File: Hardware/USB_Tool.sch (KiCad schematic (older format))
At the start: 57 parts, among them J1 USB_B_Micro, P1 RED, P2 RGB, P3 Green, P4 Green, P5 Blue, P6 Green, P7 Green, P8 Blue, SW1 SW_2TO1, U1 MRF89XAM8A, U2 NCP114, U3 MCP2221A, U4 PIC18F46K40_44, X1 EXTENDER_SPI_1, X10 Extension, X11 EXTENDER_LED_1, X12 CONN_ICSP, X2 EXTENDER_IO_2, X3 EXTENDER_IO_1, X4 EXTENDER_POWER_2, X5 EXTENDER_POWER_1, X6 Extender_I2C_1, X7 Extender_I2C_2, X9 Extension

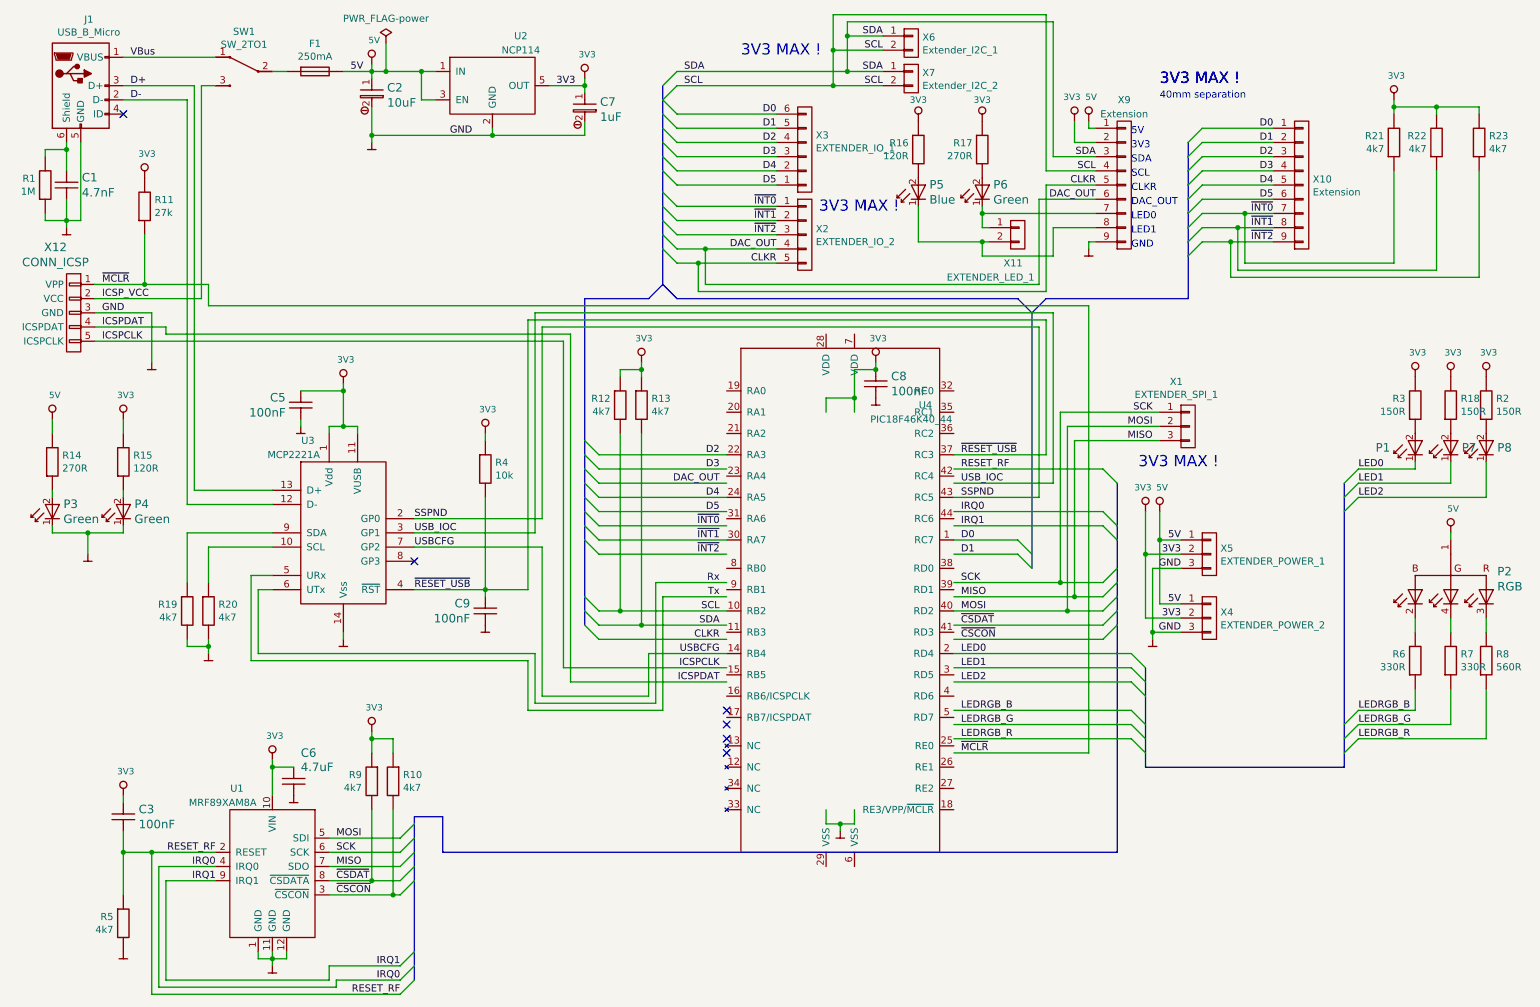
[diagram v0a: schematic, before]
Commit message: 1
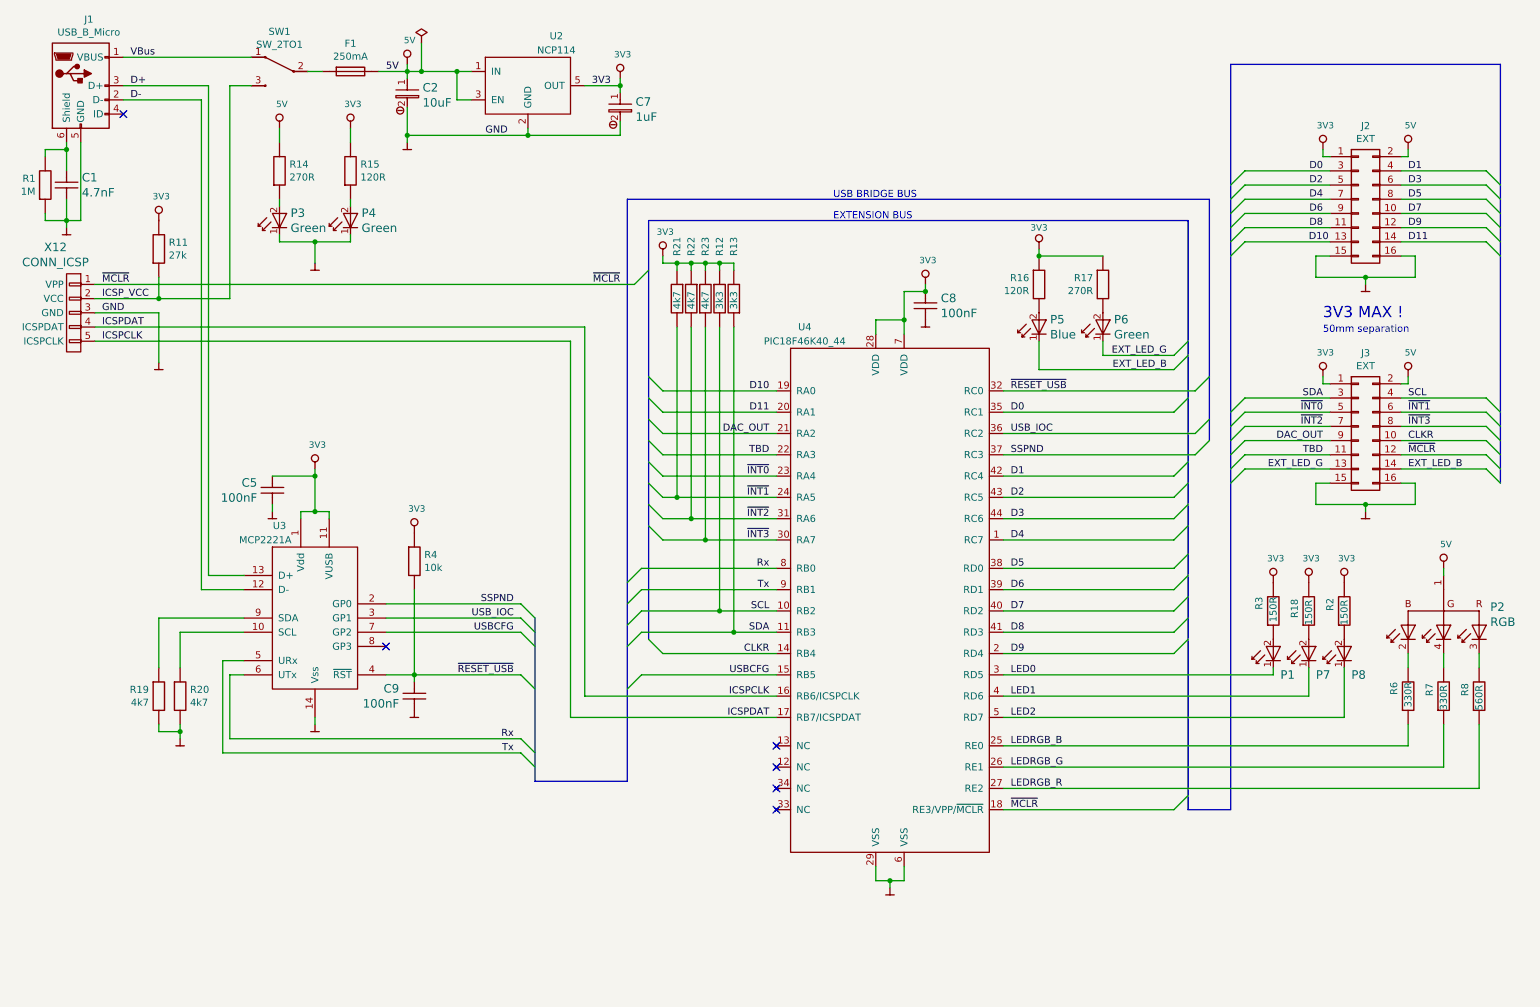
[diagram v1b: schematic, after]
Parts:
- removed C3: 100nF, 0EsseivaN_Lib:C_1206_HandSoldering, symbol 0EsseivaN_Lib:CAPA
- removed C6: 4.7uF, 0EsseivaN_Lib:C_0805_HandSoldering, symbol 0EsseivaN_Lib:CAPA
- removed R10, R5, R9: 4k7, 0EsseivaN_Lib:R_0603_HandSoldering, symbol 0EsseivaN_Lib:R
- removed U1: MRF89XAM8A, 0EsseivaN_Lib:MRF89XAM8A, symbol 0EsseivaN_Lib:MRF89XAM8A
- removed X1: EXTENDER_SPI_1, 0EsseivaN_Lib:CH_03P, symbol 0EsseivaN_Lib:CONN_01X03
- removed X10, X9: Extension, 0EsseivaN_Lib:Pin_Header_Straight_1x09_Pitch2.54mm, symbol 0EsseivaN_Lib:CONN_01X09
- removed X11: EXTENDER_LED_1, 0EsseivaN_Lib:CH_02P, symbol 0EsseivaN_Lib:CONN_01X02
- removed X2: EXTENDER_IO_2, 0EsseivaN_Lib:CH_05P, symbol 0EsseivaN_Lib:CONN_01X05
- removed X3: EXTENDER_IO_1, 0EsseivaN_Lib:CH_06P, symbol 0EsseivaN_Lib:CONN_01X06
- removed X4: EXTENDER_POWER_2, 0EsseivaN_Lib:CH_03P, symbol 0EsseivaN_Lib:CONN_01X03
- removed X5: EXTENDER_POWER_1, 0EsseivaN_Lib:CH_03P, symbol 0EsseivaN_Lib:CONN_01X03
- removed X6: Extender_I2C_1, 0EsseivaN_Lib:CH_02P, symbol 0EsseivaN_Lib:CONN_01X02
- removed X7: Extender_I2C_2, 0EsseivaN_Lib:CH_02P, symbol 0EsseivaN_Lib:CONN_01X02
- added J2, J3: EXT, symbol 0EsseivaN_Lib:Conn_02x08_Odd_Even
- R12, R13: value 4k7 -> 3k3
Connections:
- net labels added: D10, D11, D6, D7, D8, D9, EXT_LED_B, EXT_LED_G, TBD, ~INT3
- net labels removed: IRQ0, IRQ1, MISO, MOSI, RESET_RF, SCK, ~CSCON, ~CSDAT
- wire segments 323 -> 217
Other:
- note added: "50mm separation"
- note added: "EXTENSION BUS"
- note added: "USB BRIDGE BUS"
- note removed: "3V3"
- note removed: "40mm separation"
- note removed: "5V"
- note removed: "CLKR"
- note removed: "DAC_OUT"
- note removed: "GND"
- note removed: "LED0"
- note removed: "LED1"
- note removed: "SCL"
- note removed: "SDA"
- moved on the sheet: C2, C5, C7, C8, C9, F1, P1, P2, P3, P4, P5, P6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
